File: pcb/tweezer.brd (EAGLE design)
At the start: 20 x 26 mm, 37 parts, among them IC1 AD7995, IC2 TS507CLT, IC3 TS507CLT, IC5 ESDA6V1SC5, IC6 AT24CS04-SOT23

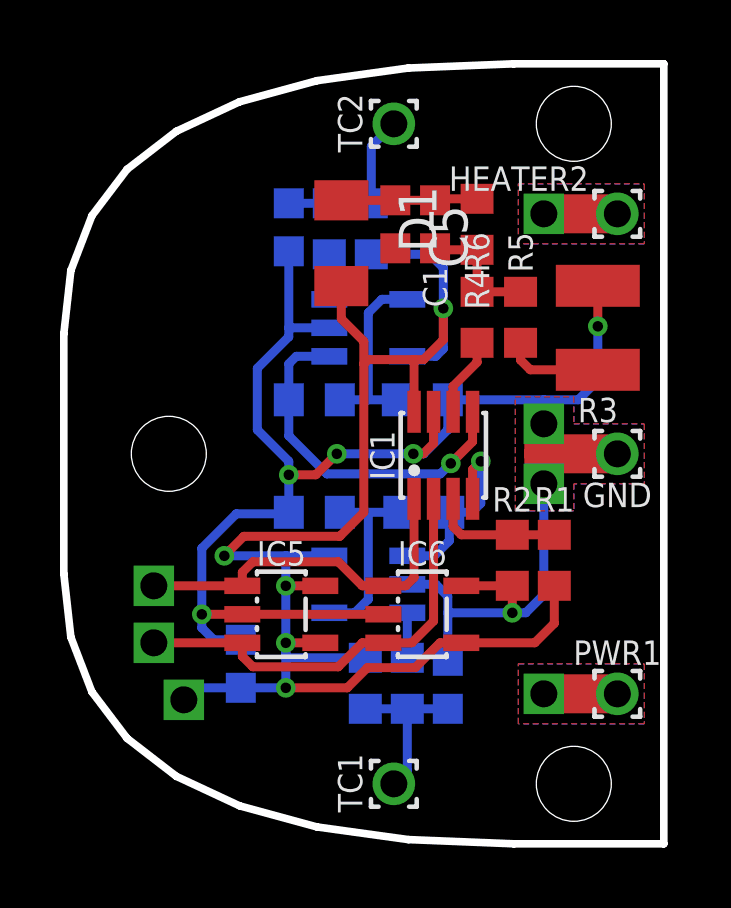
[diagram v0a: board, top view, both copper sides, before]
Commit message: boms reworked
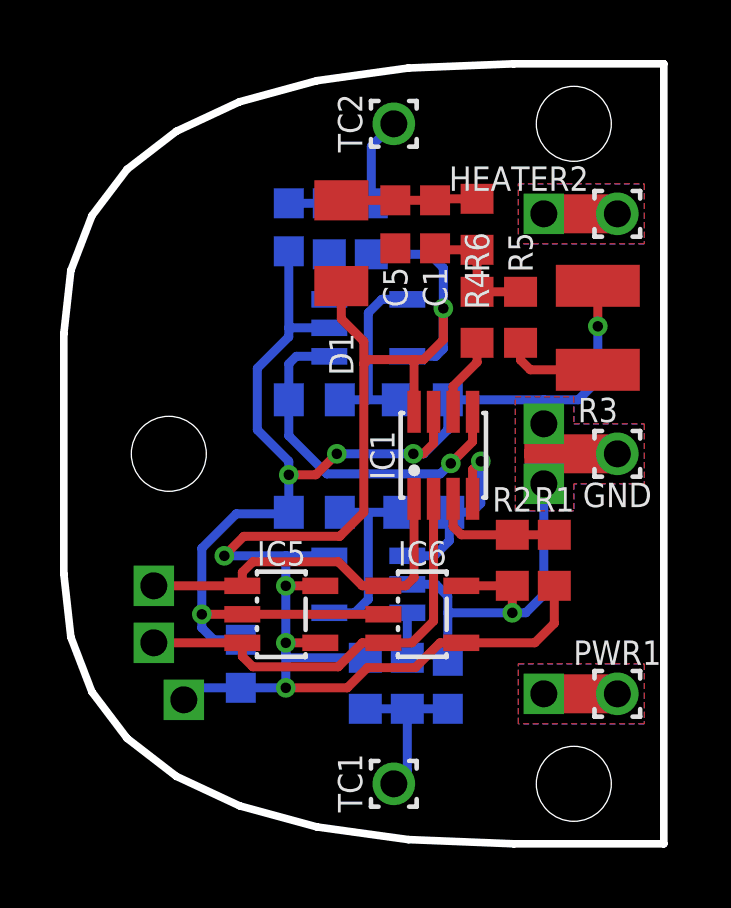
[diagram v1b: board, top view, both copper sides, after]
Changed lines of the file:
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@@
 <?xml version="1.0" encoding="utf-8"?>
 <!DOCTYPE eagle SYSTEM "eagle.dtd">
-<eagle version="9.4.2">
+<eagle version="9.5.0">
 <drawing>
 <settings>
@@
 <layer number="14" name="Route14" color="1" fill="6" visible="no" active="no"/>
 <layer number="15" name="Route15" color="4" fill="6" visible="no" active="no"/>
-<layer number="16" name="Bottom" color="1" fill="1" visible="yes" active="yes"/>
+<layer number="16" name="Bottom" color="1" fill="1" visible="no" active="yes"/>
 <layer number="17" name="Pads" color="2" fill="1" visible="yes" active="yes"/>
 <layer number="18" name="Vias" color="2" fill="1" visible="yes" active="yes"/>
@@
 <layer number="20" name="Dimension" color="24" fill="1" visible="yes" active="yes"/>
 <layer number="21" name="tPlace" color="7" fill="1" visible="yes" active="yes"/>
-<layer number="22" name="bPlace" color="7" fill="1" visible="yes" active="yes"/>
+<layer number="22" name="bPlace" color="7" fill="1" visible="no" active="yes"/>
 <layer number="23" name="tOrigins" color="15" fill="1" visible="yes" active="yes"/>
-<layer number="24" name="bOrigins" color="15" fill="1" visible="yes" active="yes"/>
-<layer number="25" name="tNames" color="7" fill="1" visible="no" active="yes"/>
+<layer number="24" name="bOrigins" color="15" fill="1" visible="no" active="yes"/>
+<layer number="25" name="tNames" color="7" fill="1" visible="yes" active="yes"/>
 <layer number="26" name="bNames" color="7" fill="1" visible="no" active="yes"/>
 <layer number="27" name="tValues" color="7" fill="1" visible="no" active="yes"/>
@@
 <layer number="38" name="bTest" color="7" fill="1" visible="no" active="yes"/>
 <layer number="39" name="tKeepout" color="4" fill="11" visible="yes" active="yes"/>
-<layer number="40" name="bKeepout" color="1" fill="11" visible="yes" active="yes"/>
-<layer number="41" name="tRestrict" color="4" fill="10" visible="no" active="yes"/>
+<layer number="40" name="bKeepout" color="1" fill="11" visible="no" active="yes"/>
+<layer number="41" name="tRestrict" color="4" fill="10" visible="yes" active="yes"/>
 <layer number="42" name="bRestrict" color="1" fill="10" visible="no" active="yes"/>
-<layer number="43" name="vRestrict" color="2" fill="10" visible="no" active="yes"/>
+<layer number="43" name="vRestrict" color="2" fill="10" visible="yes" active="yes"/>
 <layer number="44" name="Drills" color="7" fill="1" visible="no" active="yes"/>
 <layer number="45" name="Holes" color="7" fill="1" visible="yes" active="yes"/>
@@
 </element>
 <element name="D1" library="solderpi" library_urn="urn:adsk.eagle:library:1437534" package="SOD123-F" package3d_urn="urn:adsk.eagle:package:1609183/2" value="BAT54H" x="9.25" y="20.02" smashed="yes" rot="R270">
-<attribute name="NAME" x="11.155" y="21.925" size="1.27" layer="25" rot="R270"/>
+<attribute name="NAME" x="9.25" y="17.0216" size="0.8128" layer="25" rot="R90" align="center-right"/>
 <attribute name="OC_DIGIKEY" value="1727-3569-1-ND" x="9.25" y="20.02" size="1.778" layer="27" rot="R270" display="off"/>
 <attribute name="VALUE" x="6.075" y="21.925" size="1.27" layer="27" rot="R270"/>
 </element>
 <element name="C4" library="common" library_urn="urn:adsk.eagle:library:8241912" package="C0603" package3d_urn="urn:adsk.eagle:package:8241929/3" value="1µF" x="5.9" y="6" smashed="yes" rot="MR90">
-<attribute name="NAME" x="7.035" y="5.365" size="1.27" layer="26" rot="MR90"/>
+<attribute name="NAME" x="5.9" y="4.5746" size="0.8128" layer="26" rot="MR90" align="center-right"/>
 <attribute name="OC_DIGIKEY" value="1276-1034-1-ND" x="5.9" y="6" size="1.778" layer="28" rot="MR90" display="off"/>
 <attribute name="VALUE" x="3.695" y="5.365" size="1.27" layer="28" rot="MR90"/>
 </element>
 <element name="C5" library="common" library_urn="urn:adsk.eagle:library:8241912" package="C0603" package3d_urn="urn:adsk.eagle:package:8241929/3" value="1µF" x="11.05" y="20.65" smashed="yes" rot="R270">
-<attribute name="NAME" x="12.185" y="21.285" size="1.27" layer="25" rot="R270"/>
+<attribute name="NAME" x="11.05" y="19.2246" size="0.8128" layer="25" rot="R90" align="center-right"/>
 <attribute name="OC_DIGIKEY" value="1276-1034-1-ND" x="11.05" y="20.65" size="1.778" layer="27" rot="R270" display="off"/>
 <attribute name="VALUE" x="8.845" y="21.285" size="1.27" layer="27" rot="R270"/>
